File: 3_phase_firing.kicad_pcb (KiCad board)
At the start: 2 copper layers, 142.5 x 77.5 mm, 67 parts, among them J1 IN1, J2 IN2, J3 OUT, J4 USB_B, J5 Conn_01x03, J6 Conn_01x02, J7 Conn_01x03, J8 Conn_01x02, Q1 MMBT3904, Q2 MMBT3904, Q3 MMBT3904, Q4 MMBT3904, Q5 MMBT3904, Q6 MMBT3904, U1 LM339, U10 4N35, U11 4N35, U12 4N35, U2 L7812, U3 4N35, U4 4N35, U5 4N35, U6 YAAJ_WeAct_BlackPill_Part_Like, U7 4N35, U8 4N35, U9 4N35

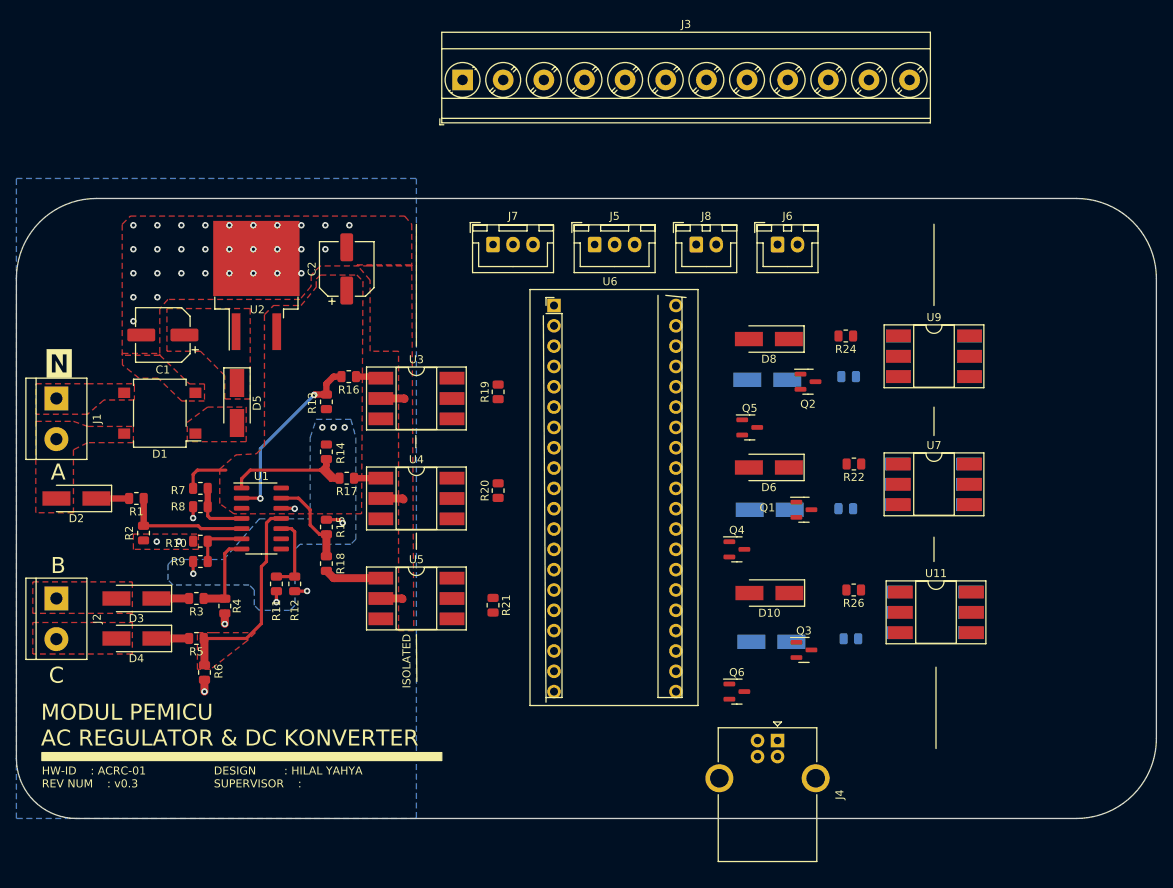
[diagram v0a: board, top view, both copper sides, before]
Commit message: done with all revision
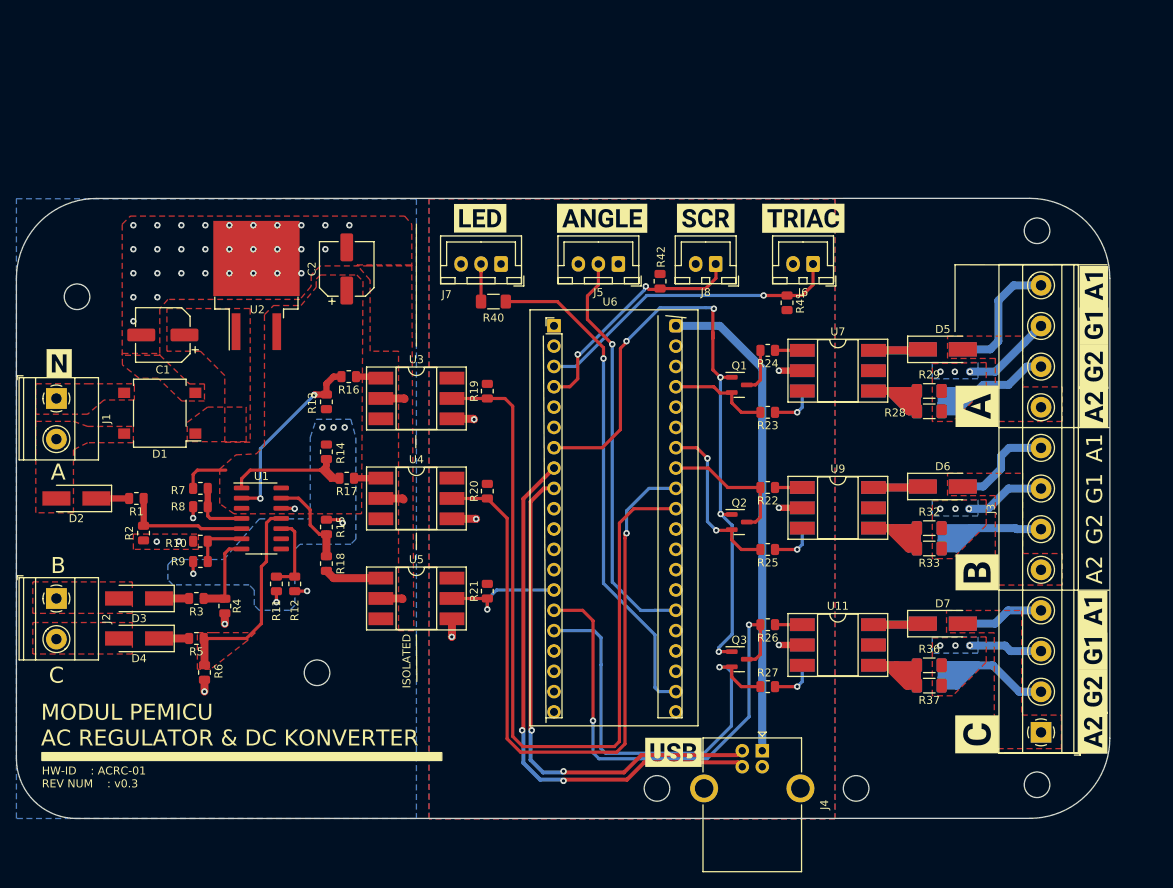
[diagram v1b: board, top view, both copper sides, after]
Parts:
- removed D11: 1N4007, Diode_SMD:D_SMA_Handsoldering
- removed Q4, Q5, Q6: MMBT3904, Package_TO_SOT_SMD:SOT-23
- added R28: 1K, Resistor_SMD:R_1206_3216Metric_Pad1.30x1.75mm_HandSolder, F.Cu at (186.6, 69.1)
- added R29: 1K, Resistor_SMD:R_1206_3216Metric_Pad1.30x1.75mm_HandSolder, F.Cu at (186.6, 66.6)
- added R30: 1K, Resistor_SMD:R_1206_3216Metric_Pad1.30x1.75mm_HandSolder, B.Cu at (186.6, 69.1)
- added R31: 1K, Resistor_SMD:R_1206_3216Metric_Pad1.30x1.75mm_HandSolder, B.Cu at (186.6, 66.6)
- added R32: 1K, Resistor_SMD:R_1206_3216Metric_Pad1.30x1.75mm_HandSolder, F.Cu at (186.6, 83.7)
- added R33: 1K, Resistor_SMD:R_1206_3216Metric_Pad1.30x1.75mm_HandSolder, F.Cu at (186.6, 86.2)
- added R34: 1K, Resistor_SMD:R_1206_3216Metric_Pad1.30x1.75mm_HandSolder, B.Cu at (186.6, 83.7)
- added R35: 1K, Resistor_SMD:R_1206_3216Metric_Pad1.30x1.75mm_HandSolder, B.Cu at (186.6, 86.2)
- added R36: 1K, Resistor_SMD:R_1206_3216Metric_Pad1.30x1.75mm_HandSolder, F.Cu at (186.6, 100.9)
- added R37: 1K, Resistor_SMD:R_1206_3216Metric_Pad1.30x1.75mm_HandSolder, F.Cu at (186.6, 103.4)
- added R38: 1K, Resistor_SMD:R_1206_3216Metric_Pad1.30x1.75mm_HandSolder, B.Cu at (186.6, 100.9)
- added R39: 1K, Resistor_SMD:R_1206_3216Metric_Pad1.30x1.75mm_HandSolder, B.Cu at (186.6, 103.4)
- added R40: 220, Resistor_SMD:R_1206_3216Metric_Pad1.30x1.75mm_HandSolder, F.Cu at (132.1, 55.4)
- added R41: 10K, Resistor_SMD:R_0805_2012Metric, F.Cu at (168.8, 55.5)
- added R42: 10K, Resistor_SMD:R_0805_2012Metric, F.Cu at (153.0, 52.8)
- added REF**: MountingHole_3.2mm_M3, MountingHole:MountingHole_3.2mm_M3, F.Cu at (177.5, 116.2)
- added REF**: MountingHole_3.2mm_M3, MountingHole:MountingHole_3.2mm_M3, F.Cu at (80.1, 54.8)
- added REF**: MountingHole_3.2mm_M3, MountingHole:MountingHole_3.2mm_M3, F.Cu at (152.6, 116.2)
- added REF**: MountingHole_3.2mm_M3, MountingHole:MountingHole_3.2mm_M3, F.Cu at (200.1, 46.5)
- added REF**: MountingHole_3.2mm_M3, MountingHole:MountingHole_3.2mm_M3, F.Cu at (110.1, 101.8)
- added REF**: MountingHole_3.2mm_M3, MountingHole:MountingHole_3.2mm_M3, F.Cu at (200.1, 115.8)
- added kibuzzard-63D8BD9F: G***, kibuzzard-63D8BD9F, F.Cu at (154.6, 111.7)
- added kibuzzard-63DA9566: G***, kibuzzard-63DA9566, F.Cu at (207.2, 58.4)
- added kibuzzard-63DA9566: G***, kibuzzard-63DA9566, F.Cu at (207.1, 99.1)
- added kibuzzard-63DA95C1: G***, kibuzzard-63DA95C1, F.Cu at (192.6, 68.5)
- added kibuzzard-63DA9616: G***, kibuzzard-63DA9616, F.Cu at (192.6, 109.5)
- added kibuzzard-63DA961C: G***, kibuzzard-63DA961C, F.Cu at (192.6, 89.2)
- added kibuzzard-63DA96B7: G***, kibuzzard-63DA96B7, F.Cu at (207.2, 68.6)
- added kibuzzard-63DA96B7: G***, kibuzzard-63DA96B7, F.Cu at (207.1, 109.2)
- added kibuzzard-63DA974B: G***, kibuzzard-63DA974B, F.Cu at (207.2, 63.5)
- added kibuzzard-63DA974B: G***, kibuzzard-63DA974B, F.Cu at (207.1, 104.2)
- added kibuzzard-63DA9751: G***, kibuzzard-63DA9751, F.Cu at (207.2, 53.5)
- added kibuzzard-63DA9751: G***, kibuzzard-63DA9751, F.Cu at (207.1, 94.2)
- added kibuzzard-63DA9A23: G***, kibuzzard-63DA9A23, F.Cu at (170.9, 45.0)
- added kibuzzard-63DA9A91: G***, kibuzzard-63DA9A91, F.Cu at (158.7, 45.0)
- added kibuzzard-63DA9AA3: G***, kibuzzard-63DA9AA3, F.Cu at (145.7, 45.0)
- added kibuzzard-63DA9AAF: G***, kibuzzard-63DA9AAF, F.Cu at (130.5, 45.0)
- D10, D8: moved to B.Cu
- D7: moved to F.Cu
- J1, J2: footprint TerminalBlock:TerminalBlock_bornier-2_P5.08mm -> TerminalBlock_Phoenix:TerminalBlock_Phoenix_MKDS-1,5-2-5.08_1x02_P5.08mm_Horizontal
- J3: value OUT -> OUTPUT; footprint TerminalBlock_Phoenix:TerminalBlock_Phoenix_MKDS-3-12-5.08_1x12_P5.08mm_Horizontal -> TerminalBlock_Phoenix:TerminalBlock_Phoenix_MKDS-1,5-12-5.08_1x12_P5.08mm_Horizontal
- J5: value Conn_01x03 -> KNOB_ANGLE
- J6: value Conn_01x02 -> TRIAC_BUTTON_CONN
- J7: value Conn_01x03 -> LED_CONN
- J8: value Conn_01x02 -> SCR_BUTTON_CONN
- R22, R24, R26: value 2K2 -> 220
- R23, R25, R27: value 2K2 -> 220; moved to F.Cu
- U10, U11, U12, U7, U8, U9: value 4N35 -> MOC3021M
- U6: value YAAJ_WeAct_BlackPill_Part_Like -> STM32F401CCU6
- moved J3 109.0 mm to (200.6, 109.2), turned to 90 degrees
- moved D5 88.5 mm to (188.3, 61.4), turned to 0 degrees
- moved D7 25.9 mm to (188.3, 95.6), turned to 0 degrees
- moved D9 25.7 mm to (188.3, 78.5), turned to 0 degrees
- moved R25 23.9 mm to (166.4, 86.4)
- moved U10 22.4 mm to (175.2, 81.2)
- moved U9 22.4 mm to (175.2, 81.2)
- moved D10 22.0 mm to (188.3, 95.6), turned to 0 degrees
- moved D6 21.9 mm to (188.3, 78.5), turned to 0 degrees
- moved D8 21.8 mm to (188.3, 61.4), turned to 0 degrees
- moved Q2 19.5 mm to (162.9, 82.9)
- moved U7 18.6 mm to (175.2, 64.0)
- moved U8 18.5 mm to (175.2, 64.0)
- moved Q1 17.6 mm to (162.9, 65.8)
- moved R23 15.5 mm to (166.4, 69.2)
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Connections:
- D1 pad 1: /DB_OUT -> /DB_D_OUT
- D10 pad 2: GATE_C1 -> LOAD_C
- D5 pad 1: /DB_D_OUT -> Net-(D5-Pad1)
- D5 pad 2: /DB_OUT -> A
- D6 pad 2: GATE_B1 -> B
- D7 pad 2: GATE_B2 -> C
- D8 pad 2: GATE_A1 -> LOAD_A
- D9 pad 2: GATE_A2 -> LOAD_B
- J3 pad 1: OUTC2_E -> C
- J3 pad 10: OUTA2_C -> SCR_G2_A
- J3 pad 11: OUTA1_E -> SCR_G1_A
- J3 pad 12: OUTA1_C -> LOAD_A
- J3 pad 2: OUTC2_C -> SCR_G2_C
- J3 pad 3: OUTC1_E -> SCR_G1_C
- J3 pad 4: OUTC1_C -> LOAD_C
- J3 pad 5: OUTB2_E -> B
- J3 pad 6: OUTB2_C -> SCR_G2_B
- J3 pad 7: OUTB1_E -> SCR_G1_B
- J3 pad 8: OUTB1_C -> LOAD_B
- J3 pad 9: OUTA2_E -> A
- J4 pad 1: unconnected-(J4-Pad1) -> +5V
- J4 pad 2: unconnected-(J4-Pad2) -> USB-
- J4 pad 3: unconnected-(J4-Pad3) -> USB+
- J4 pad 4: unconnected-(J4-Pad4) -> GND
- J7 pad 2: LED_INDICATOR_1 -> Net-(J7-Pad2)
- Q1 pad 1: TRIAC_MODE -> MODE_SELECT
- Q1 pad 2: Net-(D7-Pad1) -> GATE_A2
- Q1 pad 3: Net-(D6-Pad1) -> GATE_A1
- Q2 pad 1: TRIAC_MODE -> MODE_SELECT
- Q2 pad 2: Net-(D9-Pad1) -> GATE_B2
- Q2 pad 3: Net-(D8-Pad1) -> GATE_B1
- Q3 pad 1: TRIAC_MODE -> MODE_SELECT
- Q3 pad 2: Net-(D11-Pad1) -> GATE_C2
- Q3 pad 3: Net-(D10-Pad1) -> GATE_C1
- R22 pad 2: Net-(D6-Pad1) -> GATE_B1
- R23 pad 2: Net-(D7-Pad1) -> GATE_A2
- R24 pad 2: Net-(D8-Pad1) -> GATE_A1
- R25 pad 2: Net-(D9-Pad1) -> GATE_B2
- R26 pad 2: Net-(D10-Pad1) -> GATE_C1
- R27 pad 2: Net-(D11-Pad1) -> GATE_C2
- U10 pad 4: OUTA2_E -> Net-(D9-Pad1)
- U10 pad 5: OUTA2_C -> unconnected-(U10-Pad5)
- U10 pad 6: unconnected-(U10-Pad6) -> Net-(R34-Pad2)
- U11 pad 4: OUTC1_E -> Net-(R36-Pad2)
- U11 pad 5: OUTC1_C -> unconnected-(U11-Pad5)
- U11 pad 6: unconnected-(U11-Pad6) -> Net-(D7-Pad1)
- U12 pad 4: OUTC2_E -> Net-(D10-Pad1)
- U12 pad 5: OUTC2_C -> unconnected-(U12-Pad5)
- U12 pad 6: unconnected-(U12-Pad6) -> Net-(R38-Pad2)
- U6 pad 37: unconnected-(U6-Pad37) -> GATE_A2
- U6 pad 40: unconnected-(U6-Pad40) -> +5V
- U6 pad 7: GATE_A2 -> MODE_SELECT
- U6 pad 8: unconnected-(U6-Pad8) -> USB+
- U6 pad 9: unconnected-(U6-Pad9) -> USB-
- U7 pad 1: Net-(R22-Pad1) -> Net-(R24-Pad1)
- U7 pad 4: OUTB1_E -> Net-(R28-Pad2)
- U7 pad 5: OUTB1_C -> unconnected-(U7-Pad5)
- U7 pad 6: unconnected-(U7-Pad6) -> Net-(D5-Pad1)
- U8 pad 4: OUTB2_E -> Net-(D8-Pad1)
- U8 pad 5: OUTB2_C -> unconnected-(U8-Pad5)
- U8 pad 6: unconnected-(U8-Pad6) -> Net-(R30-Pad2)
- U9 pad 1: Net-(R24-Pad1) -> Net-(R22-Pad1)
- U9 pad 4: OUTA1_E -> Net-(R32-Pad2)
- U9 pad 5: OUTA1_C -> unconnected-(U9-Pad5)
- U9 pad 6: unconnected-(U9-Pad6) -> Net-(D6-Pad1)
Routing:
- net ZCD_A: track 0.00 -> 98.5 mm
- net ZCD_B: track 0.00 -> 87.9 mm, vias 0 -> 1
- net MODE_SELECT: track 0.00 -> 83.2 mm, vias 0 -> 5
- net USB+: track 0.00 -> 68.0 mm, vias 0 -> 2
- net USB-: track 0.00 -> 64.4 mm, vias 0 -> 2
- net LED_INDICATOR_1: track 0.00 -> 62.6 mm, vias 0 -> 1
- net GATE_C1: track 0.00 -> 62.5 mm, vias 0 -> 2
- net +5V: track 0.00 -> 60.8 mm
- net GATE_C2: track 0.00 -> 53.5 mm, vias 0 -> 1
- net ANGLE_CONTROL: track 0.00 -> 51.1 mm, vias 0 -> 1
- net TRIAC_MODE: track 0.00 -> 39.2 mm, vias 0 -> 1
- net SCR_G2_C: track 0.00 -> 32.7 mm
- net SCR_MODE: track 0.00 -> 29.9 mm, vias 0 -> 2
- net SCR_G2_A: track 0.00 -> 29.0 mm
- net SCR_G2_B: track 0.00 -> 28.7 mm
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- added copper zone on F.Cu, net +3.3V
- added copper zone on F.Cu, net A
- added copper zone on F.Cu, net B
- added copper zone on F.Cu, net C
- added copper zone on B.Cu, net GND
- added copper zone on B.Cu, net SCR_G1_A
- added copper zone on F.Cu, net SCR_G1_A
- added copper zone on B.Cu, net SCR_G1_B
- added copper zone on F.Cu, net SCR_G1_B
- added copper zone on B.Cu, net SCR_G1_C
- added copper zone on F.Cu, net SCR_G1_C
- removed copper zone on F.Cu, net /DB_OUT
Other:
- board size 142.5 x 77.5 mm -> 136.7 x 77.5 mm
- board text added: "A1"
- board text added: "A2"
- board text added: "G1"
- board text added: "G2"
- board text removed: "DESIGN : HILAL YAHYA SUPERVISOR :"
